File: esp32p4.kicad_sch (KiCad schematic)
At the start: 54 parts, among them U13 W25Q128JVS, U3 TLV62569DBV, U8 ESP32P4-REV0, Y3 40MHz

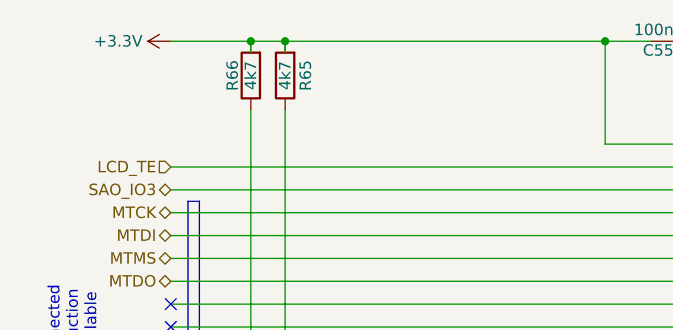
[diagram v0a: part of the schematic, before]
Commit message: Some more component placement
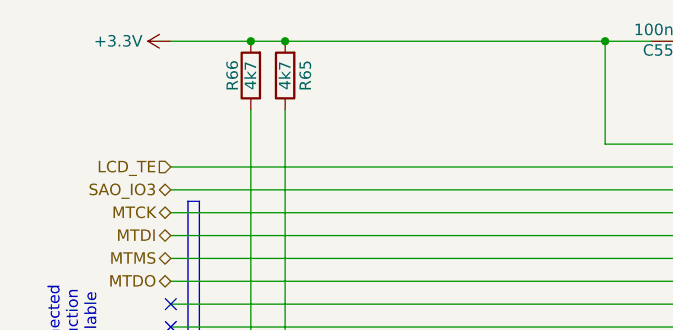
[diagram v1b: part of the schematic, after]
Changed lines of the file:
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@@
-	(wire
-		(pts
-			(xy 36.83 15.24) (xy 36.83 16.51)
-		)
-		(stroke
-			(width 0)
-			(type default)
-		)
-	)
 	(wire
 		(pts
@@
 		)
 		(stroke
-			(width 0)
-			(type default)
-		)
-	)
-	(wire
-		(pts
-			(xy 40.64 16.51) (xy 40.64 15.24)
-		)
-		(stroke
